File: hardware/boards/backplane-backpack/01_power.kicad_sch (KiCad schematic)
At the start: 28 parts, among them J1 VIN INPUT (TBD), U4 LMR51610YDBVR, U5 LMR51610YDBVR

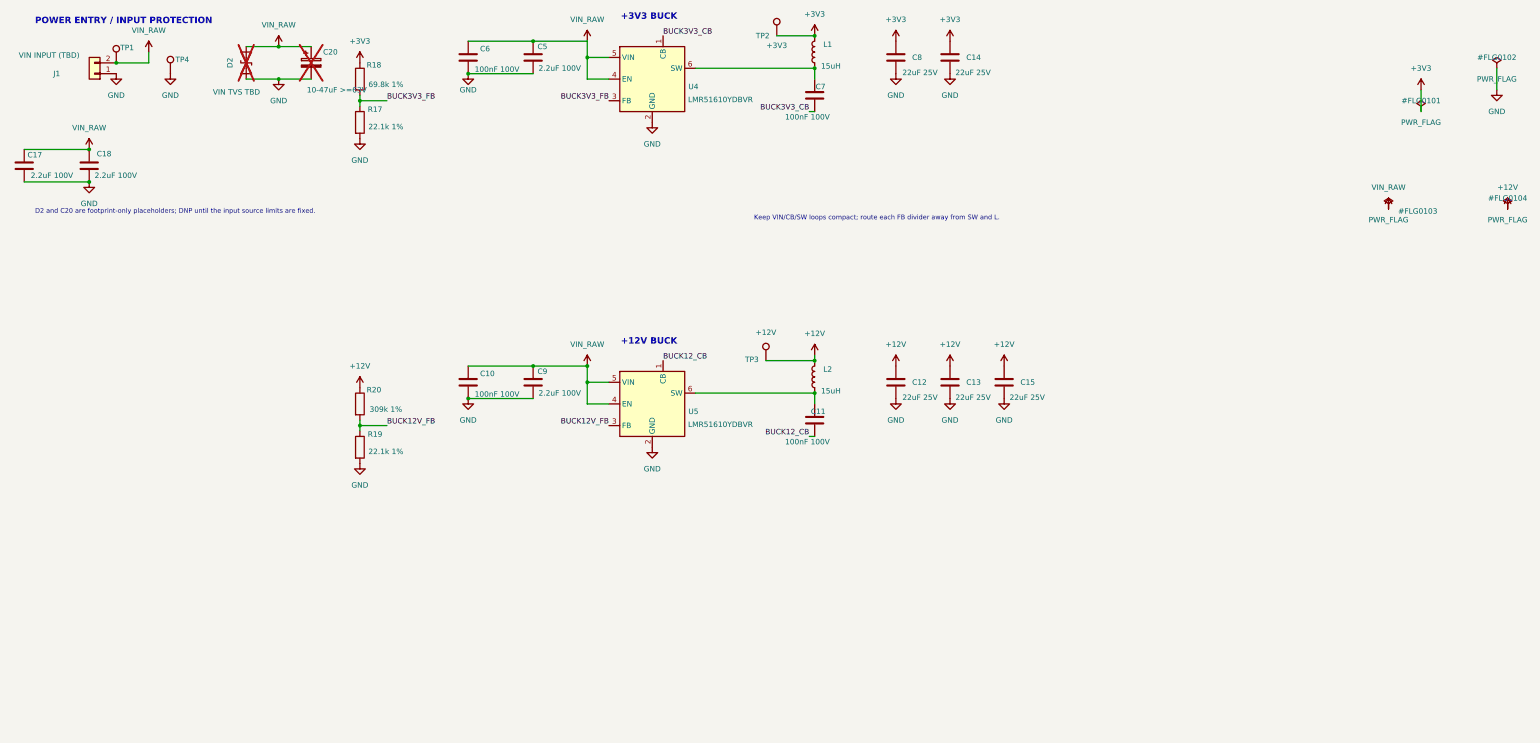
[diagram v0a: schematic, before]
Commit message: chore: checkpoint workspace changes
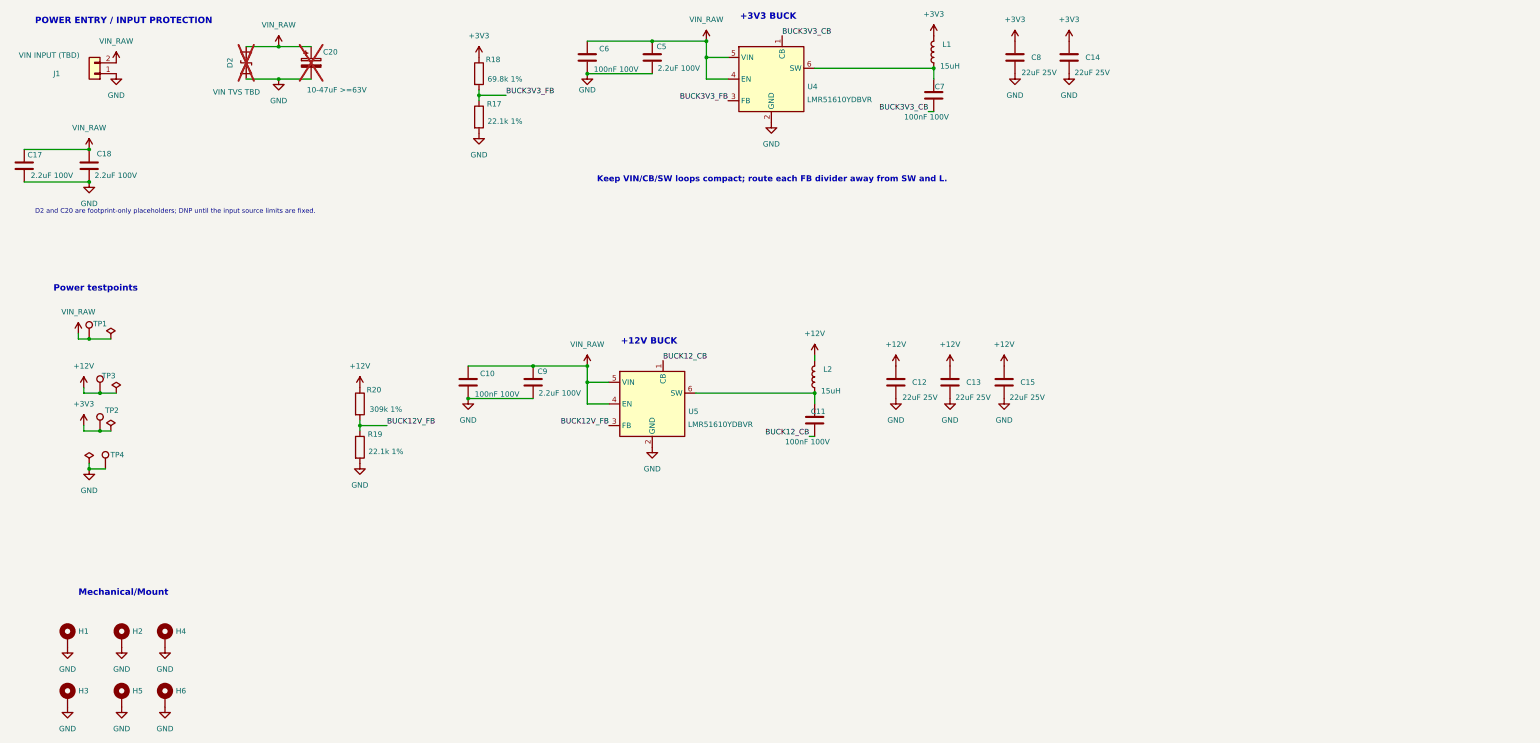
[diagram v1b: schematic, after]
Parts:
- added H1, H2, H3, H4, H5, H6: MountingHole_Pad, MountingHole:MountingHole_2.2mm_M2_Pad_Via, symbol Mechanical:MountingHole_Pad
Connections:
- net GND: now also H1.1, H2.1, H3.1, H4.1, H5.1, H6.1
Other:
- note added: "Mechanical/Mount"
- note added: "Power testpoints"
- moved on the sheet: C14, C5, C6, C7, C8, L1, R17, R18, U4
